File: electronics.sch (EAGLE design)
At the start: 21 parts, among them M1 SERVO, M2 SERVO, T1 2N3904

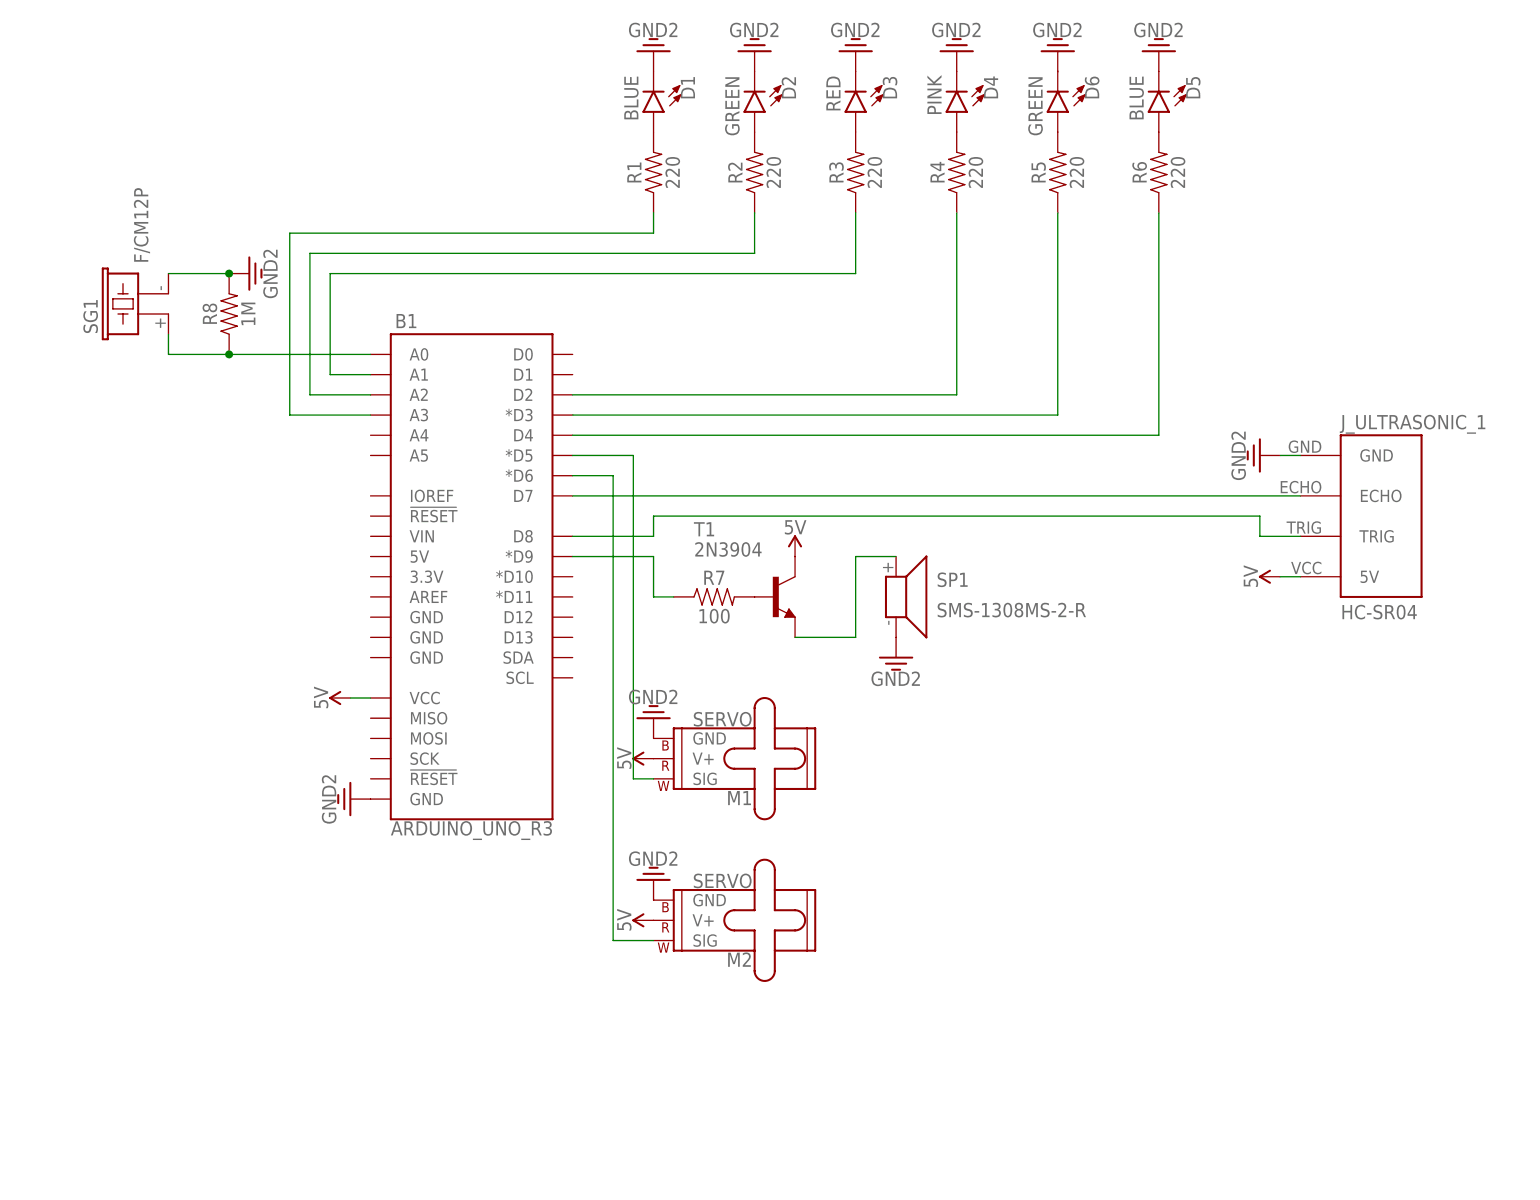
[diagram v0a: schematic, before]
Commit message: Add files via upload
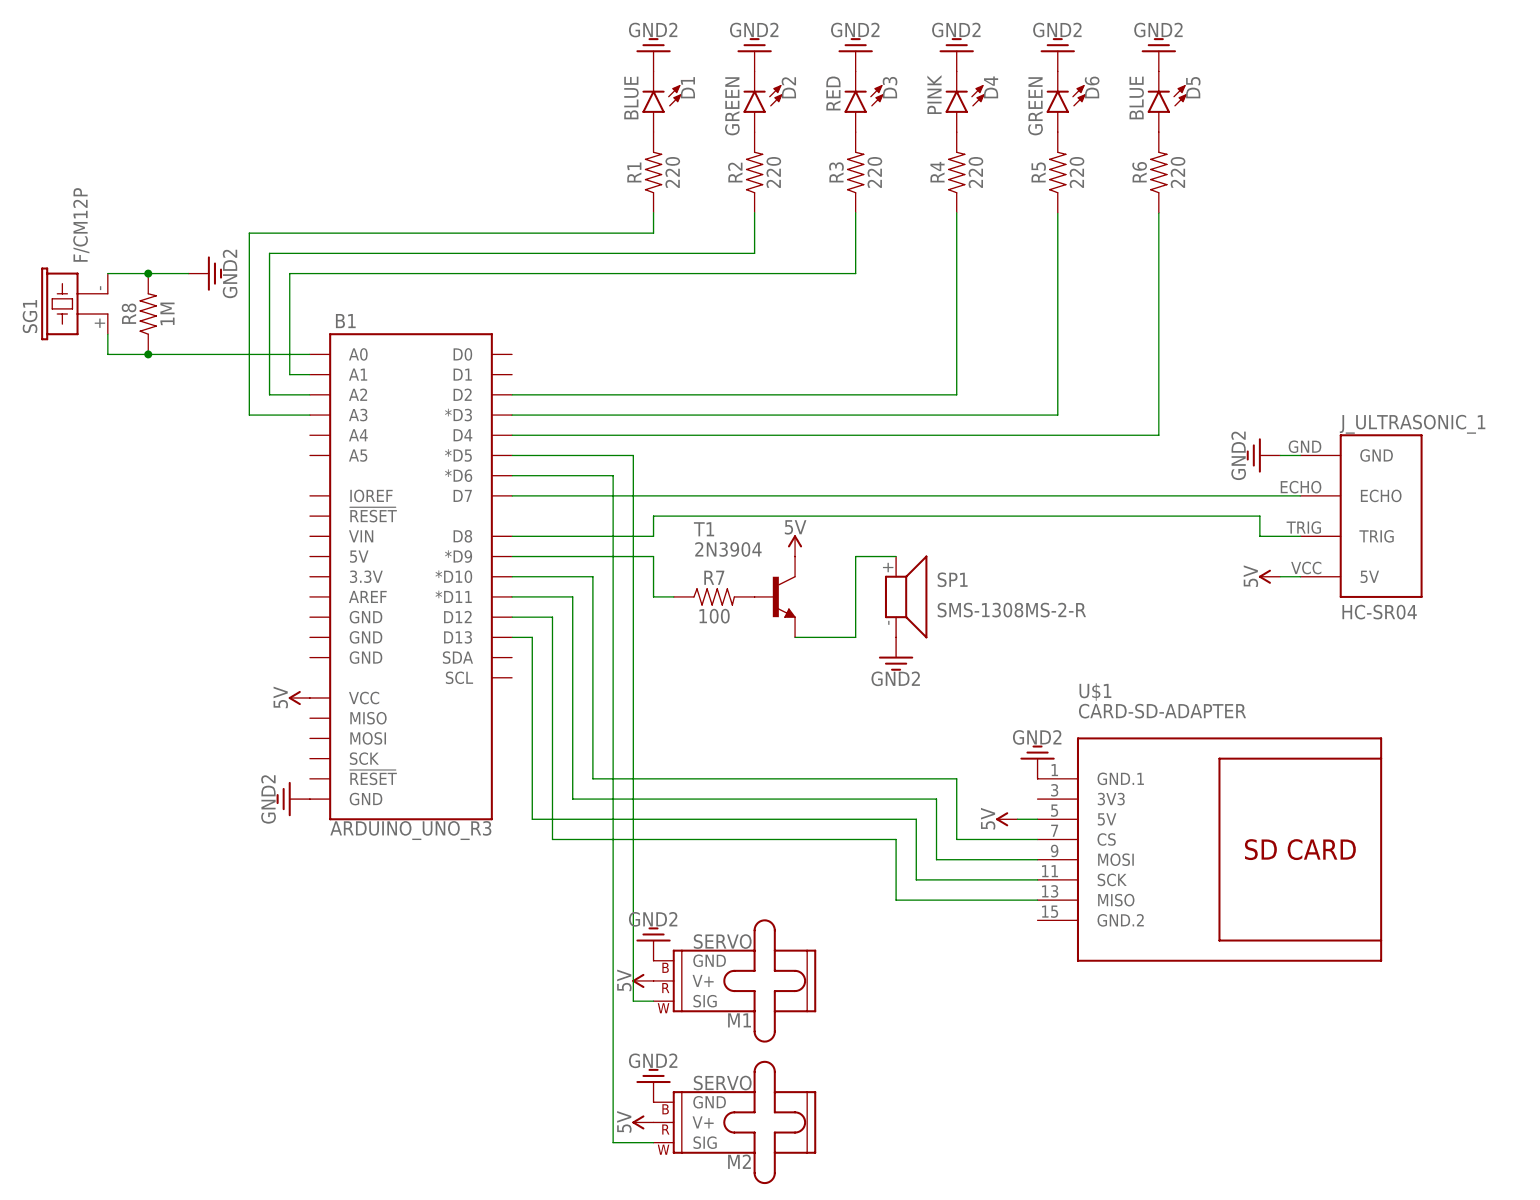
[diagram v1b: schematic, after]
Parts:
- added U$1: CARD-SD-ADAPTER, diy-modules:CARD-SD-ADAPTER
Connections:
- new net N$13: B1.*D10, U$1.CS
- new net N$22: B1.*D11, U$1.MOSI
- new net N$23: B1.D12, U$1.MISO
- new net N$24: B1.D13, U$1.SCK
- net 3.3V: now also U$1.GND.1
- net 5V: now also U$1.5V
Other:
- moved on the sheet: B1, M1, M2, R8, SG1
